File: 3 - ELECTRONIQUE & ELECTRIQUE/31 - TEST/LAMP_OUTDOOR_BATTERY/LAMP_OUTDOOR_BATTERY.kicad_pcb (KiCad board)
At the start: 2 copper layers, 15.3 x 61.6 mm, 13 parts, among them J1 629722000214, U1 MCP73833-FCI_UN, U2 MT3608

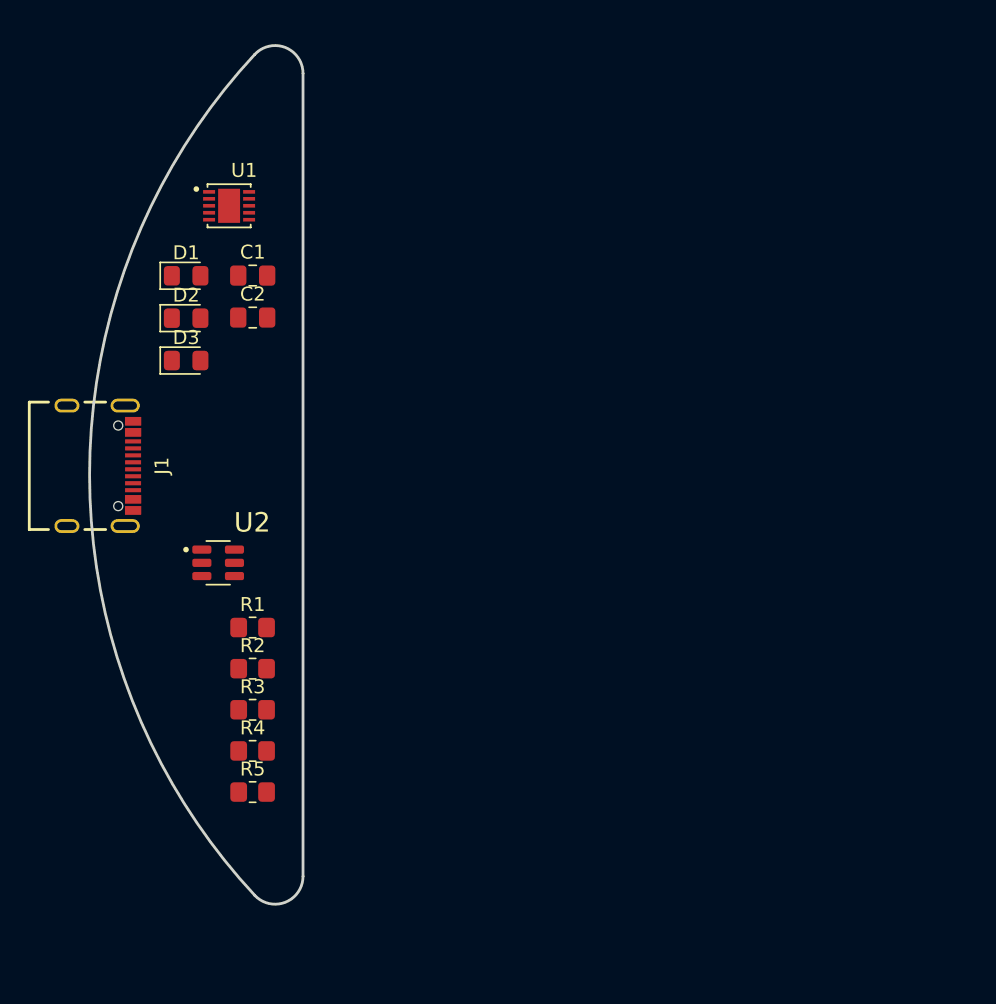
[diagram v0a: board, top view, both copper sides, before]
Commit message: Commit_1.02 Modification shape PCB
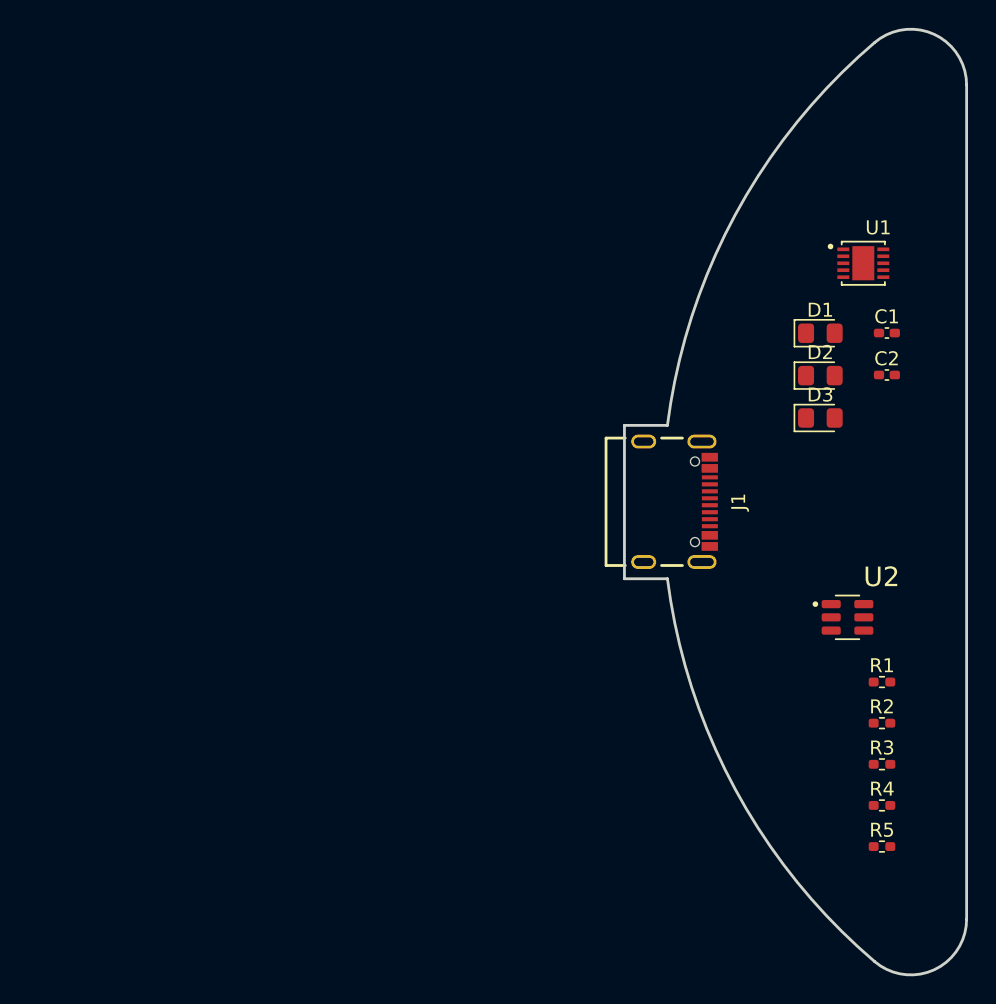
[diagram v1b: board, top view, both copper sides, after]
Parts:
- C1, C2: footprint Capacitor_SMD:C_0805_2012Metric_Pad1.18x1.45mm_HandSolder -> Capacitor_SMD:C_0402_1005Metric_Pad0.74x0.62mm_HandSolder
- R1, R2, R3, R4, R5: footprint Resistor_SMD:R_0805_2012Metric_Pad1.20x1.40mm_HandSolder -> Resistor_SMD:R_0402_1005Metric_Pad0.72x0.64mm_HandSolder
- moved C1 45.7 mm to (187.9, 79.4)
- moved C2 45.7 mm to (187.9, 82.4)
- moved D1 45.7 mm to (183.2, 79.4)
- moved D2 45.7 mm to (183.2, 82.4)
- moved D3 45.7 mm to (183.2, 85.5)
- moved U1 45.7 mm to (186.2, 74.4)
- moved R1 45.3 mm to (187.6, 104.4)
- moved R2 45.3 mm to (187.6, 107.4)
- moved R3 45.3 mm to (187.6, 110.3)
- moved R4 45.3 mm to (187.6, 113.3)
- moved R5 45.3 mm to (187.6, 116.2)
- moved U2 45.3 mm to (185.1, 99.8)
- moved J1 41.5 mm to (170.5, 91.5)
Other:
- board size 15.3 x 61.6 mm -> 24.5 x 67.8 mm
